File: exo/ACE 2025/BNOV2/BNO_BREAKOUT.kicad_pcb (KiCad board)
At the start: 2 copper layers, 67.5 x 45 mm, 17 parts, among them J2 RJ45, SW1 SW_SPDT, U1 4754, U2 PCA9615DPZ, U3 AP7361C-33E

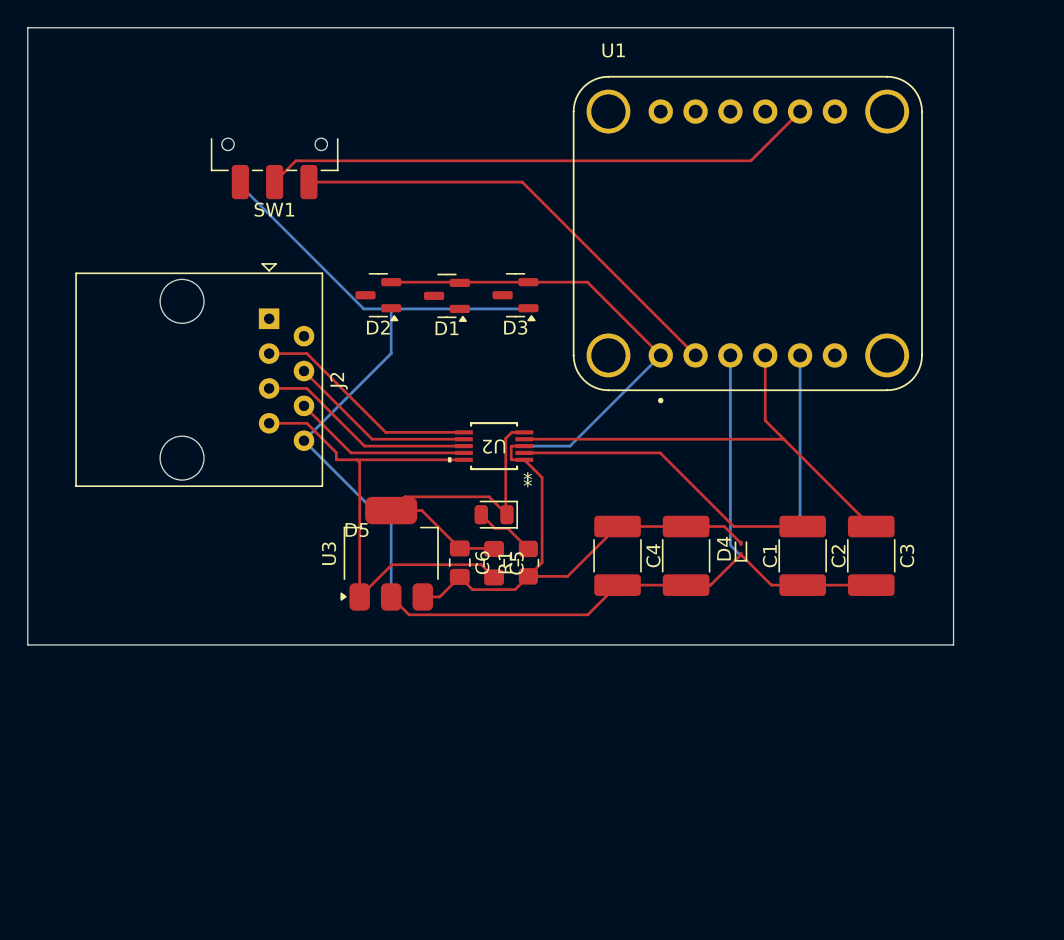
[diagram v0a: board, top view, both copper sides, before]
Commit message: BNOV2 V0.2
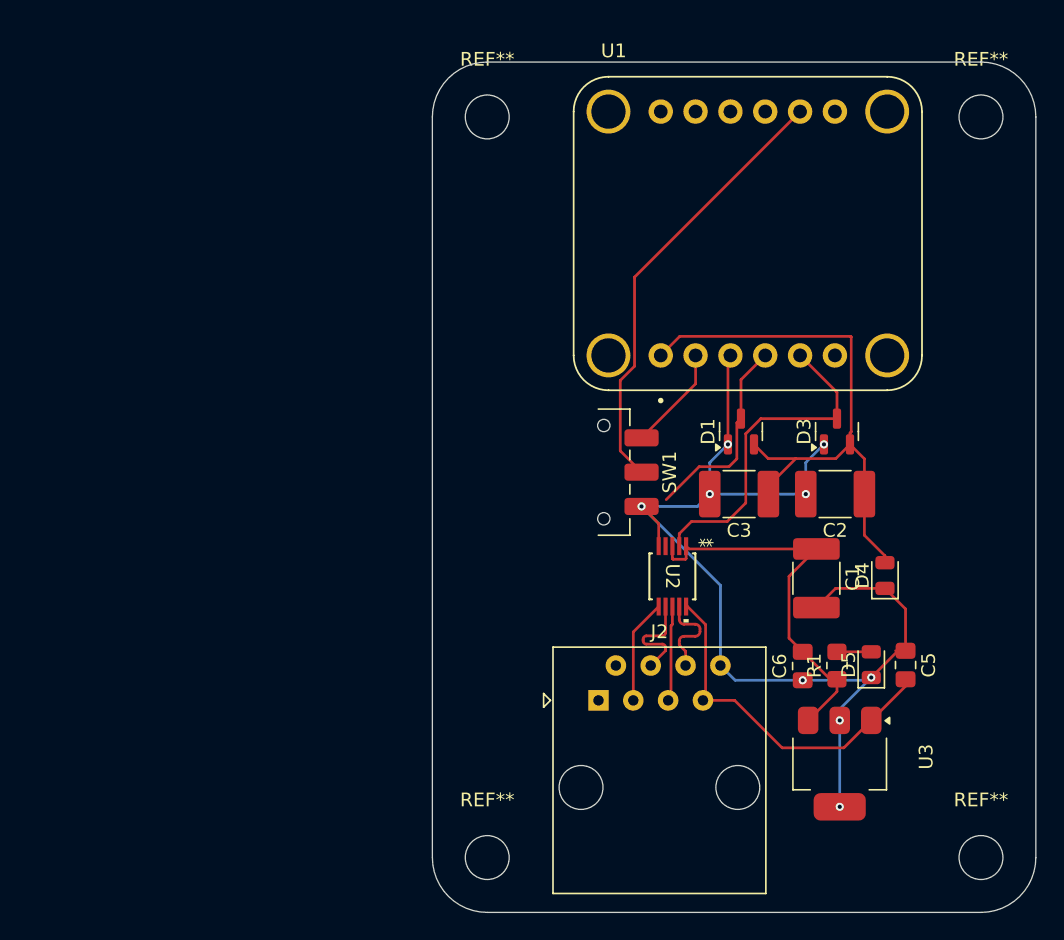
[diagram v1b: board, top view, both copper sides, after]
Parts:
- removed C4: 4.7uF, Capacitor_SMD:C_1812_4532Metric_Pad1.57x3.40mm_HandSolder
- removed D2: BAV99, Package_TO_SOT_SMD:SOT-23
- added REF**: MountingHole_3.2mm_M3, MountingHole:MountingHole_3.2mm_M3, F.Cu at (121.0, 71.5)
- added REF**: MountingHole_3.2mm_M3, MountingHole:MountingHole_3.2mm_M3, F.Cu at (157.0, 125.5)
- added REF**: MountingHole_3.2mm_M3, MountingHole:MountingHole_3.2mm_M3, F.Cu at (121.0, 125.5)
- added REF**: MountingHole_3.2mm_M3, MountingHole:MountingHole_3.2mm_M3, F.Cu at (157.0, 71.5)
- C2, C3: value 4.7uF -> 1n
- D4: value ESD9B3.3ST5G -> D_TVS_Filled; footprint Diode_SMD:D_SOD-923 -> Diode_SMD:D_0805_2012Metric
- moved J2 36.8 mm to (129.1, 114.0), turned to 0 degrees
- moved U3 36.1 mm to (146.7, 118.7), turned to -90 degrees
- moved SW1 33.9 mm to (129.5, 97.4), turned to -90 degrees
- moved C5 30.9 mm to (151.5, 111.5)
- moved D5 29.6 mm to (149.0, 111.4), turned to 90 degrees
- moved C6 26.1 mm to (144.0, 111.5), turned to 90 degrees
- moved D3 25.5 mm to (146.5, 94.4), turned to 90 degrees
- moved R1 23.7 mm to (146.5, 111.5)
- moved D1 23.6 mm to (139.5, 94.4), turned to 90 degrees
- moved U2 16.1 mm to (134.5, 105.0), turned to -90 degrees
- moved D4 10.7 mm to (150.0, 104.9)
- moved C3 10.6 mm to (139.4, 99.0), turned to 180 degrees
- moved C1 9.64 mm to (145.0, 105.1)
- moved C2 5.08 mm to (146.4, 99.0), turned to 180 degrees
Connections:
- net 5V renamed /5V
- net SCL+ renamed /SCL+
- net SCL- renamed /SCL-
- net SDA+ renamed /SDA+
- net SDA- renamed /SDA-
- C1 pad 1: 3V3 -> /3V3
- C2 pad 1: SDA -> /3V3
- C3 pad 1: SCL -> /3V3
- C6 pad 2: 3V3 -> /3V3
- D1 pad 2: 3V3 -> /3V3
- D1 pad 3: SCL -> /SCL
- D3 pad 2: 3V3 -> /3V3
- D3 pad 3: SDA -> /SDA
- D4 pad 2: 3V3 -> /3V3
- R1 pad 1: 3V3 -> /3V3
- U1 pad JP1_1: 3V3 -> /3V3
- U1 pad JP1_4: SCL -> /SCL
- U1 pad JP1_5: SDA -> /SDA
- U2 pad 1: 3V3 -> /3V3
- U2 pad 2: SDA -> /SDA
- U2 pad 3: 3V3 -> /3V3
- U2 pad 4: SCL -> /SCL
- U3 pad 3: 3V3 -> /3V3
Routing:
- net 3V3: track 73.7 -> 0.00 mm
- net /3V3: track 0.00 -> 71.7 mm
- net GND: track 131.8 -> 82.2 mm, vias 0 -> 10
- net SDA: track 35.2 -> 0.00 mm
- net SCL: track 34.6 -> 0.00 mm
- net Net-(SW1-A): track 33.4 -> 7.64 mm
- net /SDA: track 0.00 -> 24.6 mm
- net /SCL: track 0.00 -> 14.8 mm
- net /5V: track 36.8 -> 26.1 mm
- net /SCL+: track 16.6 -> 7.60 mm
- net /SDA+: track 15.9 -> 6.96 mm
- net Net-(SW1-B): track 40.4 -> 32.4 mm
- net /SDA-: track 13.1 -> 6.85 mm
- net /SCL-: track 13.7 -> 7.56 mm
- net Net-(D5-A): track 4.64 -> 2.50 mm
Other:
- board size 67.5 x 45 mm -> 44 x 62 mm
- board text removed: "DIMENSIONS DELL À CONFIRMER"
